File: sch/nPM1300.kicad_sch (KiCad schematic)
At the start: 20 parts, among them J3 USB_C_Receptacle_USB2.0_16P, J8 Conn_ARM_SWD_TagConnect_TC203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, U3 TPD3E001DRLR, U5 nRF52833-QDXX, U6 TXB0106RGY, Y2 32MHz

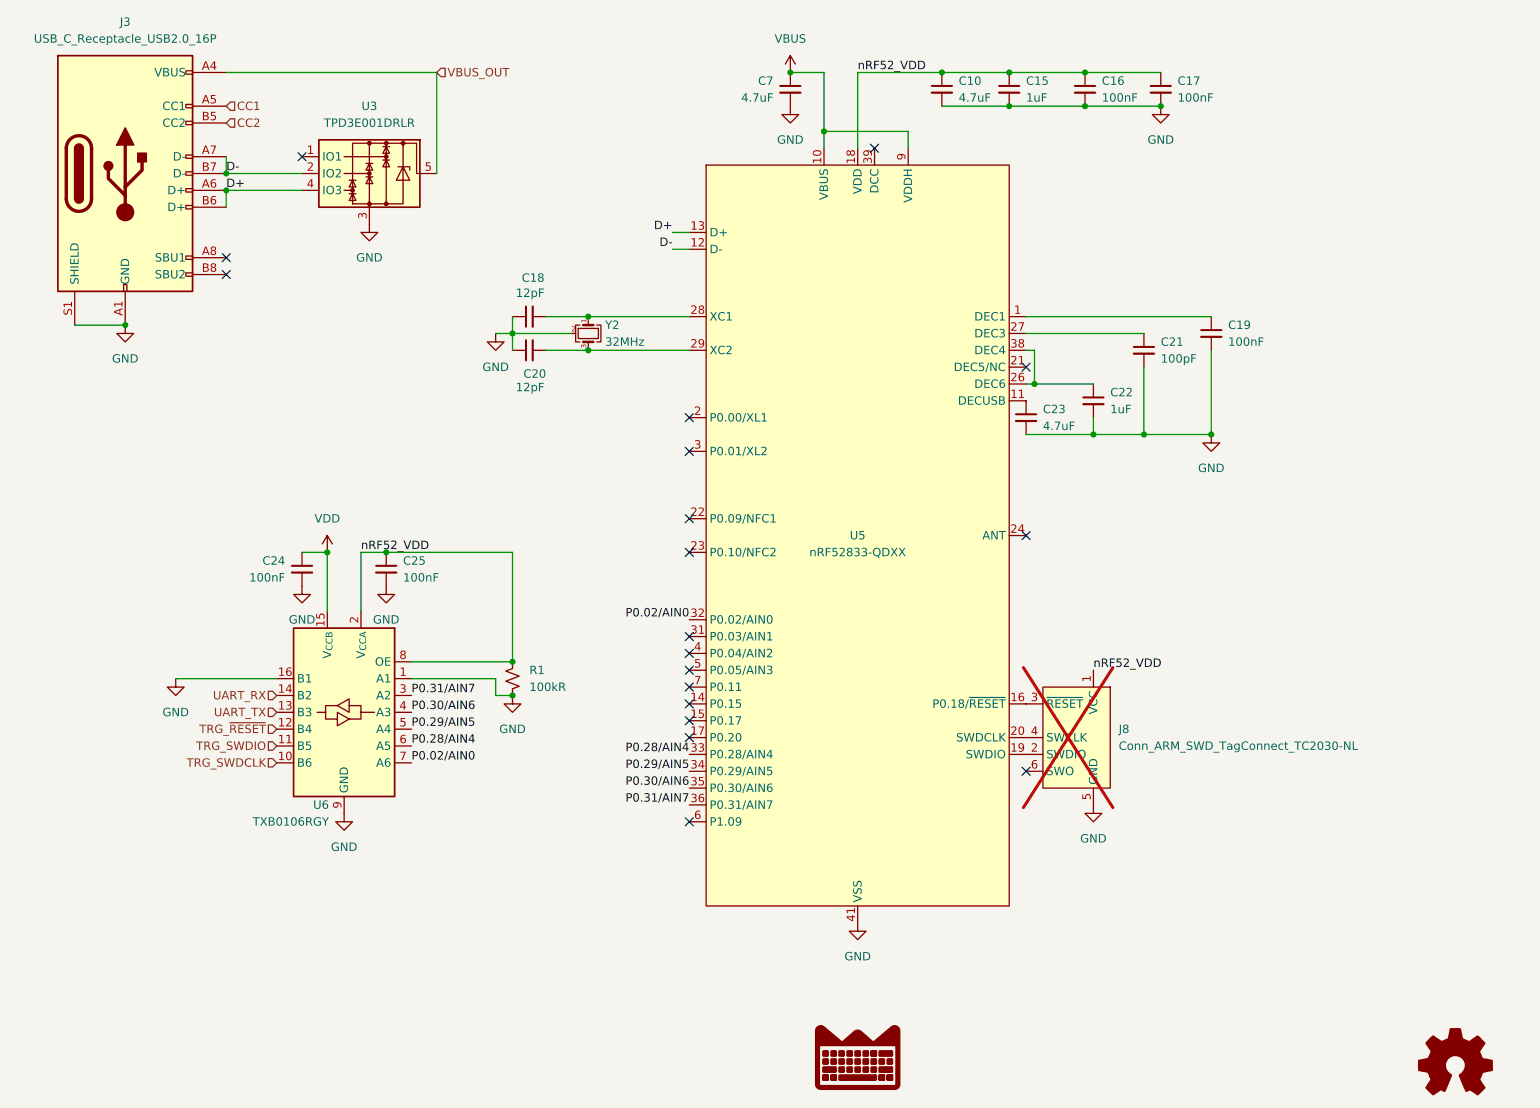
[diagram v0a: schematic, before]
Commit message: Updated 02/03/25
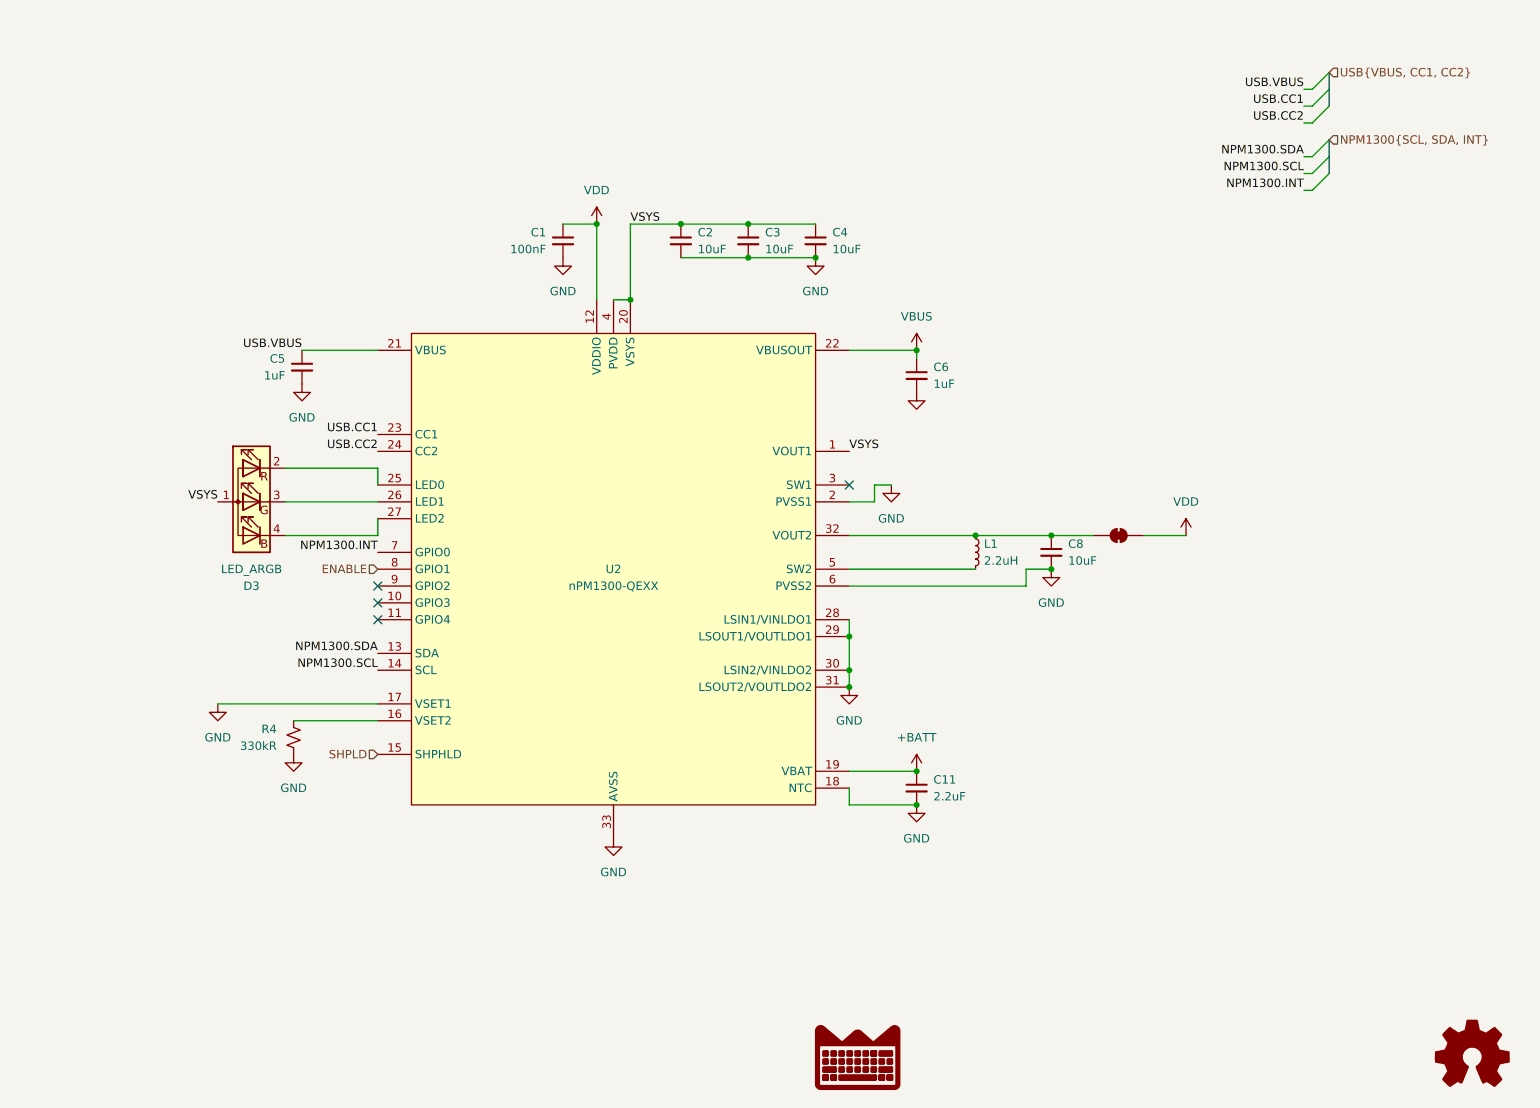
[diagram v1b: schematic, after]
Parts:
- removed C10, C23, C7: 4.7uF, Capacitor_SMD:C_0402_1005Metric, symbol Device:C_Small
- removed C15, C22: 1uF, Capacitor_SMD:C_0402_1005Metric, symbol Device:C_Small
- removed C16, C17, C19, C24, C25: 100nF, Capacitor_SMD:C_0402_1005Metric, symbol Device:C_Small
- removed C18, C20: 12pF, Capacitor_SMD:C_0402_1005Metric, symbol Device:C_Small
- removed C21: 100pF, Capacitor_SMD:C_0402_1005Metric, symbol Device:C_Small
- removed J3: USB_C_Receptacle_USB2.0_16P, marbastlib-various:USB_C_Receptacle_HRO_TYPE-C-31-M-12, symbol Connector:USB_C_Receptacle_USB2.0_16P
- removed J8: Conn_ARM_SWD_TagConnect_TC2030-NL, Connector:Tag-Connect_TC2030-IDC-NL_2x03_P1.27mm_Vertical, symbol Connector:Conn_ARM_SWD_TagConnect_TC2030-NL
- removed R1: 100kR, Resistor_SMD:R_0402_1005Metric, symbol Device:R_Small_US
- removed U3: TPD3E001DRLR, Package_TO_SOT_SMD:SOT-553, symbol Power_Protection:TPD3E001DRLR
- removed U5: nRF52833-QDXX, Package_DFN_QFN:QFN-40-1EP_5x5mm_P0.4mm_EP3.6x3.6mm_ThermalVias, symbol nordic-lib-kicad-nrf52:nRF52833-QDXX
- removed U6: TXB0106RGY, Package_DFN_QFN:Texas_RGY_R-PVQFN-N16_EP2.05x2.55mm, symbol Logic_LevelTranslator:TXB0106RGY
- removed Y2: 32MHz, Crystal:Crystal_SMD_2016-4Pin_2.0x1.6mm, symbol hlord2000-Device:Crystal_GND24_Small_EZRoute
- added C1: 100nF, Capacitor_SMD:C_0402_1005Metric, symbol Device:C_Small
- added C11: 2.2uF, Capacitor_SMD:C_0603_1608Metric, symbol Device:C_Small
- added C2, C3, C4, C8: 10uF, Capacitor_SMD:C_0603_1608Metric, symbol Device:C_Small
- added C5, C6: 1uF, Capacitor_SMD:C_0603_1608Metric, symbol Device:C_Small
- added D3: LED_ARGB, LED_SMD:LED_Wurth_150044M155260, symbol Device:LED_ARGB
- added JP1: SolderJumper_2_Bridged, Jumper:SolderJumper-2_P1.3mm_Bridged_RoundedPad1.0x1.5mm, symbol Jumper:SolderJumper_2_Bridged
- added L1: 2.2uH, Inductor_SMD:L_0603_1608Metric, symbol Device:L_Small
- added R4: 330kR, Resistor_SMD:R_0402_1005Metric, symbol Device:R_Small_US
- added U2: nPM1300-QEXX, Package_DFN_QFN:QFN-32-1EP_5x5mm_P0.5mm_EP3.6x3.6mm_ThermalVias, symbol nordic-lib-kicad-npm:nPM1300-QEXX
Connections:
- net GND: now also C1.2, C11.2, C2.2, C3.2, C4.2, C5.2, C6.2, C8.2, R4.2, U2.17 (VSET1), U2.18 (NTC), U2.2 (PVSS1), U2.28 (LSIN1/VINLDO1), U2.29 (LSOUT1/VOUTLDO1), U2.30 (LSIN2/VINLDO2), U2.31 (LSOUT2/VOUTLDO2), U2.33 (AVSS), U2.6 (PVSS2)
- net VBUS: now also C6.1, U2.22 (VBUSOUT)
- net VDD: now also C1.1, JP1.2 (B), U2.12 (VDDIO)
- new net: C8.1, JP1.1 (A), L1.1, U2.32 (VOUT2)
- new net: L1.2, U2.5 (SW2)
- new net: D3.2 (RK), U2.25 (LED0)
- new net: D3.3 (GK), U2.26 (LED1)
- new net: D3.4 (BK), U2.27 (LED2)
- new net: R4.1, U2.16 (VSET2)
- new net +BATT: C11.1, U2.19 (VBAT)
- new net ENABLE: U2.8 (GPIO1)
- new net NPM1300.INT: U2.7 (GPIO0)
- new net NPM1300.SCL: U2.14 (SCL)
- new net NPM1300.SDA: U2.13 (SDA)
- new net SHPLD: U2.15 (SHPHLD)
- new net USB.CC1: U2.23 (CC1)
- new net USB.CC2: U2.24 (CC2)
- new net USB.VBUS: C5.1, U2.21 (VBUS)
- new net VSYS: C2.1, C3.1, C4.1, D3.1 (A), U2.1 (VOUT1), U2.20 (VSYS), U2.4 (PVDD)
- no-connect marks 19 -> 4
